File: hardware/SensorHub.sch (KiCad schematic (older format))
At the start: 39 parts, among them IC1 VEML6070, IC2 LT3652EMSE, IC3 BME680, IC4 BH1726, IC5 MCP9808, M1 ParticleArgon, SW1 ENABLE, X1 WIND, X2 SOLAR

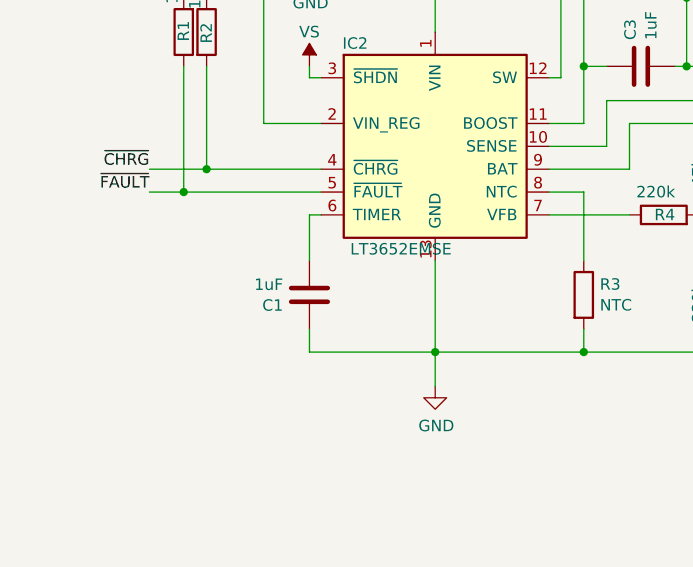
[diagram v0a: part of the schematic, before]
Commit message: Clean up hardware files
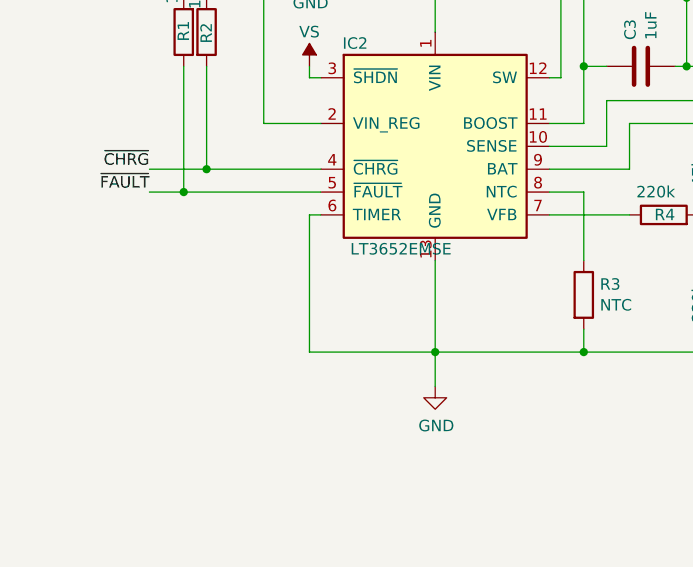
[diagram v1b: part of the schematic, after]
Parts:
- removed C1: 1uF, Capacitor_SMD:C_0805_2012Metric_Pad1.15x1.40mm_HandSolder, symbol Device:C
- IC3: Order Number 262-BME680 -> 262-BME680
- IC5: Mouser (none) -> 579-MCP9808T-E/MS
- RV1: Mfr. No. TS53YJ103MR10 -> TS53YJ103MR10
- SW1: Distributor (none) -> Mouser; Mfr. No. A6S-1104-PH -> A6S-1104-PH
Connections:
- net GND: now also IC2.6 (TIMER)
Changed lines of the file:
@@
 F 5 "BMP680" H 11121 2509 50  0001 R CNN "Mfr. No."
 F 6 "Mouser" H 11550 2600 50  0001 C CNN "Distributor"
-F 7 "262-BME680 " H 11550 2600 50  0001 C CNN "Order Number"
+F 7 "262-BME680" H 11550 2600 50  0001 C CNN "Order Number"
 	1    11550 2600
 	1    0    0    -1
@@
 F 4 "Microchip" H 9500 2650 50  0001 C CNN "Mfr."
 F 5 "MCP9808T-E/MS " H 9500 2650 50  0001 C CNN "Mfr. No."
-F 6 "" H 9500 2650 50  0001 C CNN "Mouser"
+F 6 "579-MCP9808T-E/MS " H 9500 2650 50  0001 C CNN "Mouser"
 F 7 "Mouser" H 9500 2650 50  0001 C CNN "Distributor"
 F 8 "579-MCP9808T-E/MS " H 9500 2650 50  0001 C CNN "Order Number"
@@
 F 3 "~" H 9250 6500 50  0001 C CNN
 F 4 "Omron" H 9250 6857 50  0001 C CNN "Mfr."
-F 5 "A6S-1104-PH " H 9250 6766 50  0001 C CNN "Mfr. No."
+F 5 "A6S-1104-PH" H 9250 6766 50  0001 C CNN "Mfr. No."
 F 6 "653-A6S1104PH" H 9250 6500 50  0001 C CNN "Order Number"
+F 7 "Mouser" H 9250 6500 50  0001 C CNN "Distributor"
 	1    9250 6500
 	1    0    0    -1
@@
 F 1 "10k" V 1750 2350 50  0000 R CNN
 F 2 "Potentiometer_SMD_Kampi:Potentiometer_Vishay_TS53YJ_Vertical" H 1850 2300 50  0001 C CNN
-F 3 "~" H 1850 2300 50  0001 C CNN
+F 3 "https://www.mouser.de/datasheet/2/427/ts53-1763731.pdf" H 1850 2300 50  0001 C CNN
 F 4 "Vishay" H 1780 2300 50  0001 R CNN "Mfr."
-F 5 "TS53YJ103MR10 " H 1780 2391 50  0001 R CNN "Mfr. No."
+F 5 "TS53YJ103MR10" H 1780 2391 50  0001 R CNN "Mfr. No."
 F 6 "Mouser" H 1850 2300 50  0001 C CNN "Distributor"
 F 7 "72-TS53YJ-10K " H 1850 2300 50  0001 C CNN "Order Number"
@@
 $EndComp
 Wire Wire Line
-	1850 4100 1850 4200
-Wire Wire Line
 	1850 4200 2400 4200
 Connection ~ 2400 4200
@@
 Wire Wire Line
 	1900 3600 1850 3600
-Wire Wire Line
-	1850 3600 1850 3800
 $Comp
 L Device:R R4
@@
 	1    1600 8575
 	1    0    0    1
-$EndComp
-$Comp
-L Device:C C1
-U 1 1 5EE01B4B
-P 1850 3950
-F 0 "C1" H 1965 3996 50  0000 L CNN
-F 1 "1uF" H 1965 3905 50  0000 L CNN
-F 2 "Capacitor_SMD:C_0805_2012Metric_Pad1.15x1.40mm_HandSolder" H 1888 3800 50  0001 C CNN
-F 3 "~" H 1850 3950 50  0001 C CNN
-F 4 "Kemet" H 1850 3950 50  0001 C CNN "Mfr."
-F 5 "C0805X105K3RAC3316" H 1850 3950 50  0001 C CNN "Mfr. No."
-F 6 "Mouser" H 1850 3950 50  0001 C CNN "Distributor"
-F 7 "80-C0805X105K3R3316" H 1850 3950 50  0001 C CNN "Order Number"
-	1    1850 3950
-	-1   0    0    1
 $EndComp
 $Comp
@@
 Text Notes 5450 6300 0    50   ~ 0
 The voltage divider is designed\nfor a 17.8 V solar panel.
+Wire Wire Line
+	1850 3600 1850 4200
 $EndSCHEMATC
